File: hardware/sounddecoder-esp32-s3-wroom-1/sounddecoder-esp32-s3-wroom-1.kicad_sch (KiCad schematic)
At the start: 7 parts, among them J1 Input power, U2 IS25WP256D-xM, U3 MAX98357A, U4 DRV8871DDA, U5 LM2594M-5.0, U6 AMS1117-3.3, U7 ESP32-S3-WROOM-1

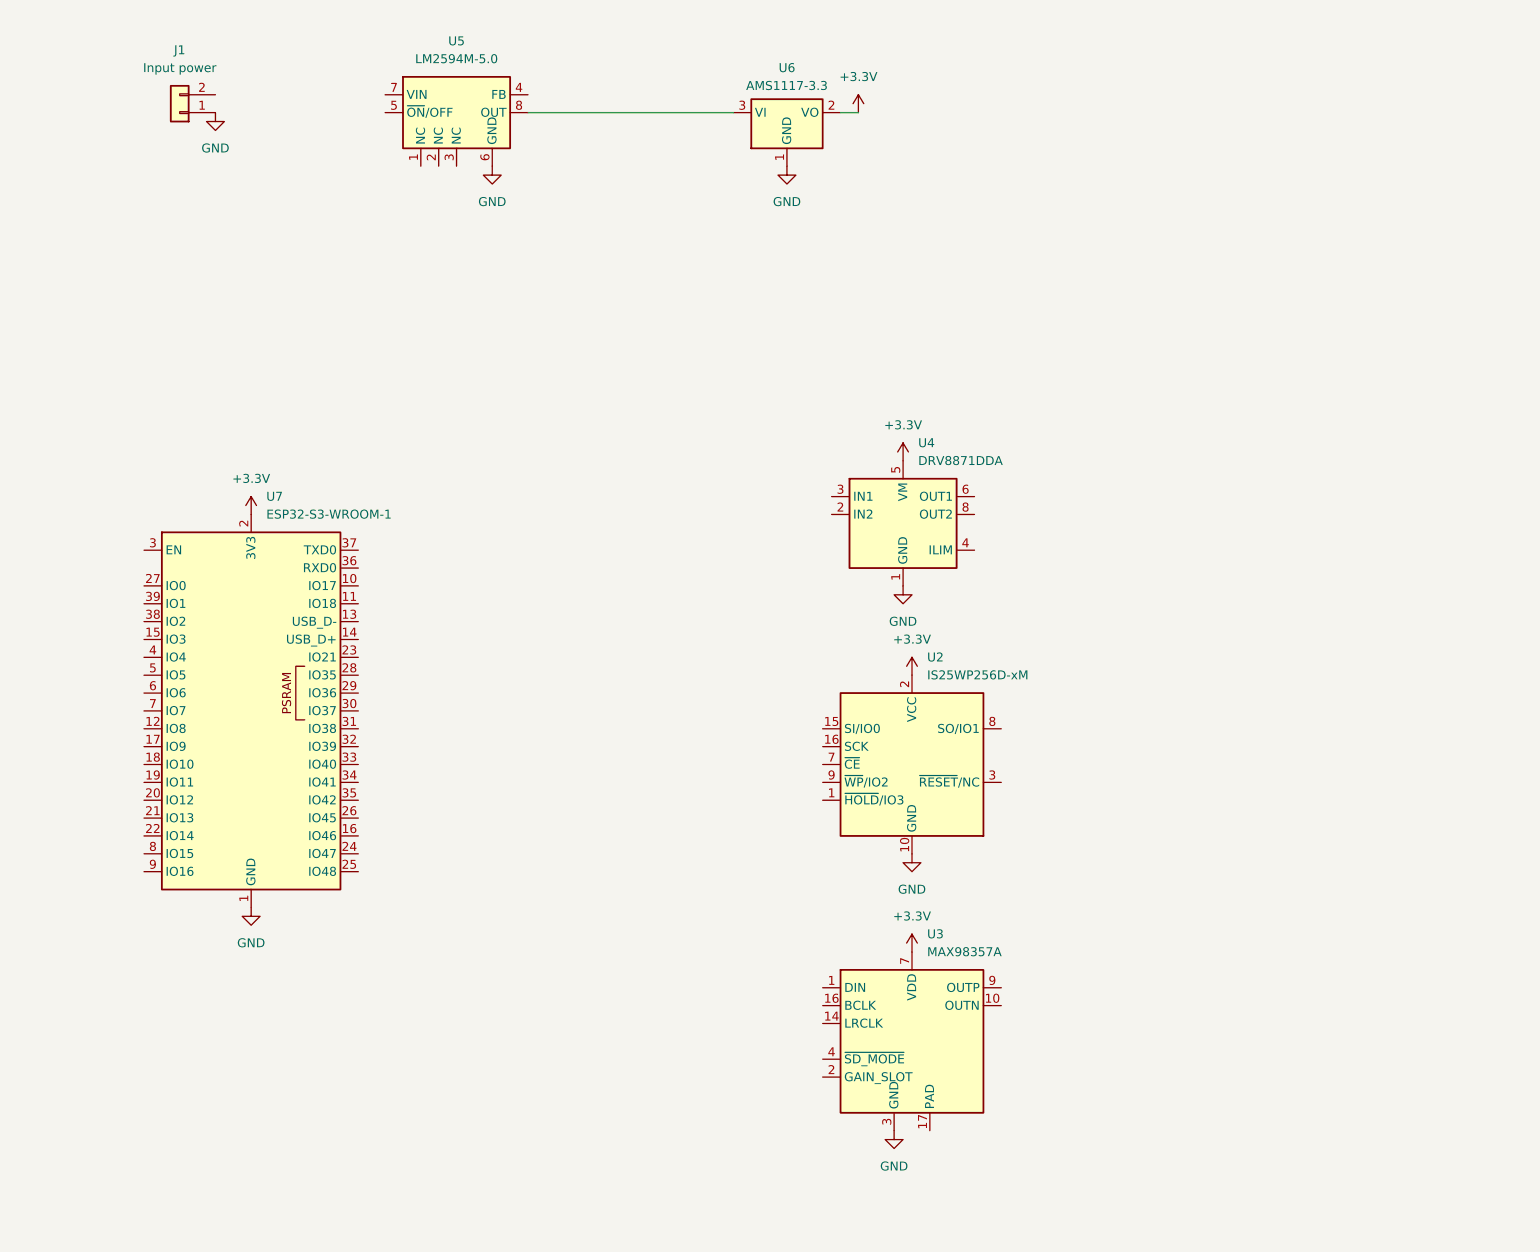
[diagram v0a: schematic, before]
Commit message: Many updates
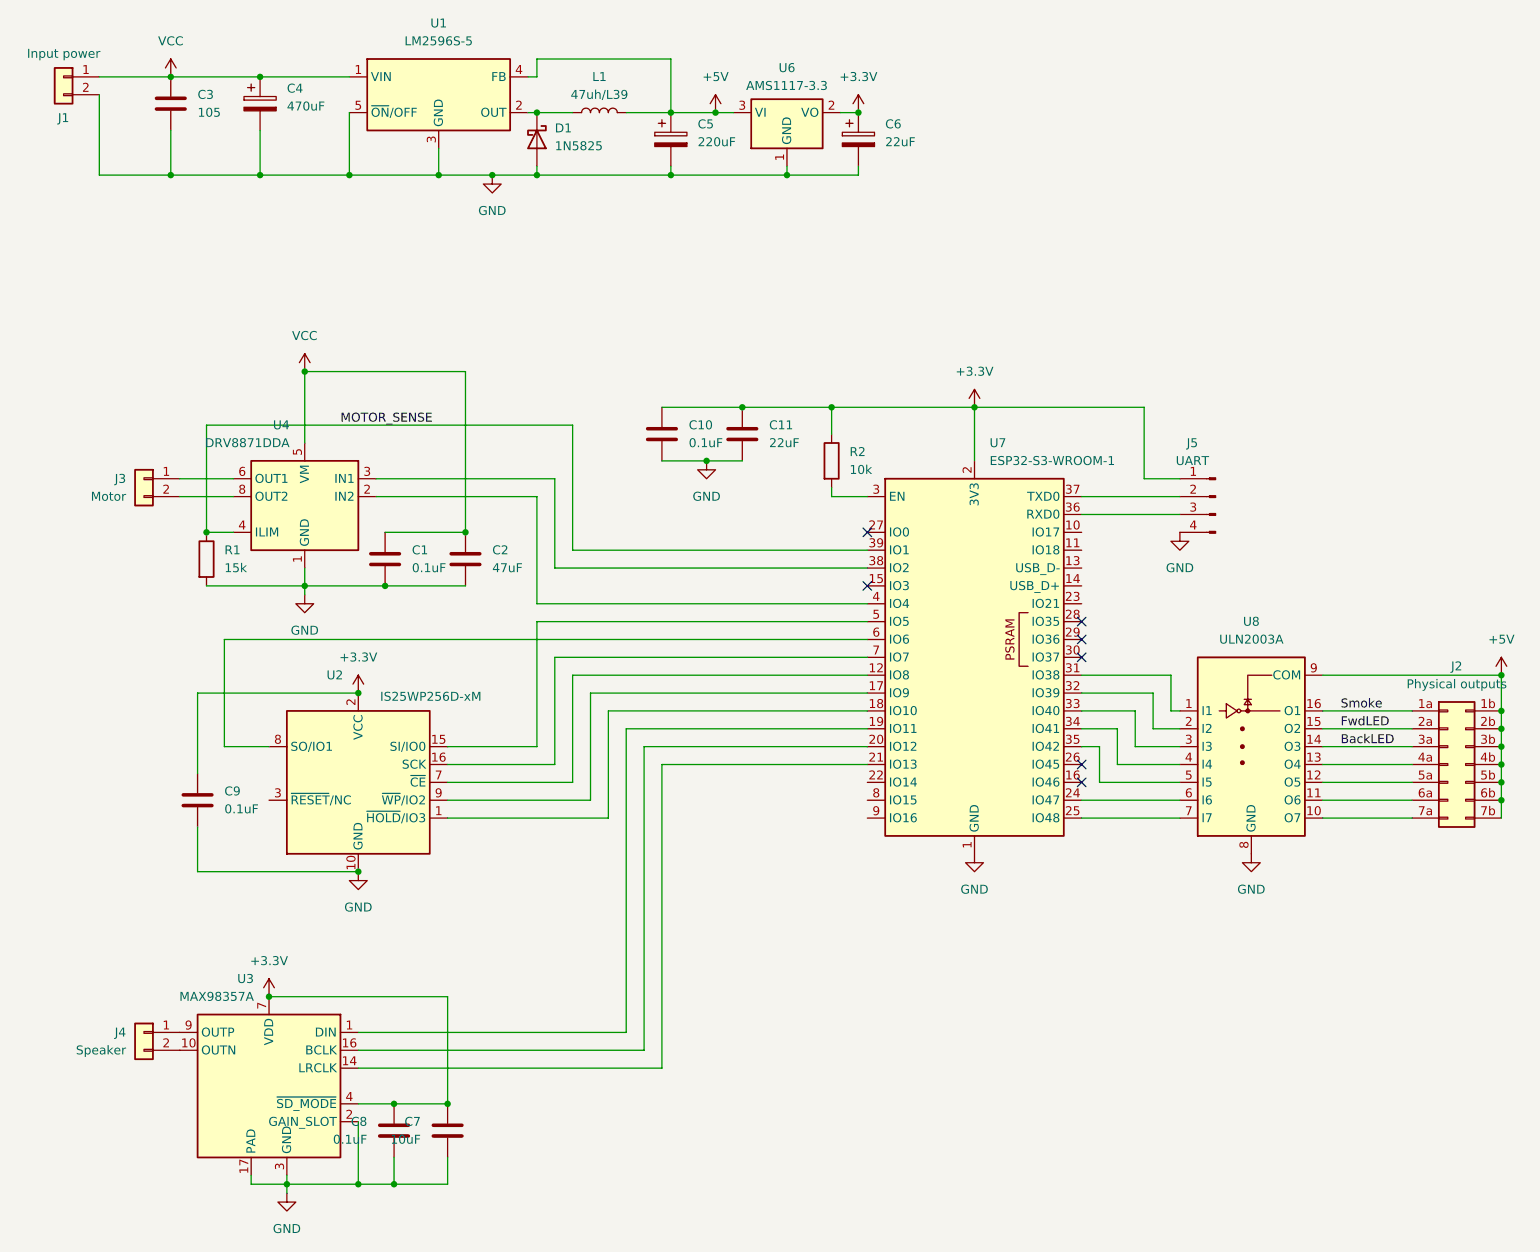
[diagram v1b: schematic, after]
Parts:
- removed U5: LM2594M-5.0, Package_SO:SOIC-8_3.9x4.9mm_P1.27mm, symbol Regulator_Switching:LM2594M-5.0
- added C1, C10, C9: 0.1uF, Capacitor_SMD:C_0805_2012Metric, symbol Device:C
- added C11: 22uF, Capacitor_SMD:C_0805_2012Metric, symbol Device:C
- added C2: 47uF, Capacitor_SMD:C_0805_2012Metric, symbol Device:C
- added C3: 105, symbol Device:C
- added C4: 470uF, symbol Device:C_Polarized
- added C5: 220uF, Capacitor_Tantalum_SMD:CP_EIA-7343-20_Kemet-V_HandSolder, symbol Device:C_Polarized
- added C6: 22uF, Capacitor_Tantalum_SMD:CP_EIA-3216-10_Kemet-I_HandSolder, symbol Device:C_Polarized
- added C7: 10uF, symbol Device:C
- added C8: 0.1uF, symbol Device:C
- added D1: 1N5825, Diode_THT:D_DO-201AD_P15.24mm_Horizontal, symbol Diode:1N5822
- added J2: Physical outputs, symbol Connector_Generic:Conn_02x07_Row_Letter_Last
- added J3: Motor, symbol Connector_Generic:Conn_01x02
- added J4: Speaker, symbol Connector_Generic:Conn_01x02
- added J5: UART, Connector_PinSocket_2.54mm:PinSocket_1x04_P2.54mm_Horizontal, symbol Connector:Conn_01x04_Pin
- added L1: 47uh/L39, Inductor_SMD:L_Bourns_SRP1245A, symbol Device:L
- added R1: 15k, symbol Device:R
- added R2: 10k, symbol Device:R
- added U1: LM2596S-5, Package_TO_SOT_SMD:TO-263-5_TabPin3, symbol Regulator_Switching:LM2596S-5
- added U8: ULN2003A, symbol Transistor_Array:ULN2003A
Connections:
- net +3.3V: now also U3.4 (~{SD_MODE}), C10.1, C11.1, C6.1, C7.1, C8.1, C9.1, J5.1 (Pin_1), R2.1; no longer U4.5 (VM)
- net GND: now also J1.2 (Pin_2), U3.17 (PAD), U3.2 (GAIN_SLOT), C1.2, C10.2, C11.2, C2.2, C3.2, C4.2, C5.2, C6.2, C7.2, C8.2, C9.2, D1.2 (A), J5.4 (Pin_4), R1.2, U1.3 (GND), U1.5 (~{ON}/OFF), U8.8 (GND); no longer J1.1 (Pin_1)
- net at U3.1 (DIN): now also U7.19 (IO11)
- net at U3.10 (OUTN): now also J4.2 (Pin_2)
- net at U3.14 (LRCLK): now also U7.21 (IO13)
- net at U3.16 (BCLK): now also U7.20 (IO12)
- net at U3.9 (OUTP): now also J4.1 (Pin_1)
- net +5V: now reaches U6.3 (VI)
- net +5V: now also C5.1, J2.1b (Pin_1b), J2.2b (Pin_2b), J2.3b (Pin_3b), J2.4b (Pin_4b), J2.5b (Pin_5b), J2.6b (Pin_6b), J2.7b (Pin_7b), L1.2, U1.4 (FB), U8.9 (COM)
- net at U7.12 (IO8): now also U2.7 (~{CE})
- net at U7.17 (IO9): now also U2.9 (~{WP}/IO2)
- net at U7.18 (IO10): now also U2.1 (~{HOLD}/IO3)
- net at U7.24 (IO47): now also U8.6 (I6)
- net at U7.25 (IO48): now also U8.7 (I7)
- net at U7.3 (EN): now also R2.2
- net at U7.31 (IO38): now also U8.1 (I1)
- net at U7.32 (IO39): now also U8.2 (I2)
- net at U7.33 (IO40): now also U8.3 (I3)
- net at U7.34 (IO41): now also U8.4 (I4)
- net at U7.35 (IO42): now also U8.5 (I5)
- net at U7.36 (RXD0): now also J5.3 (Pin_3)
- net at U7.37 (TXD0): now also J5.2 (Pin_2)
- net at U7.38 (IO2): now also U4.3 (IN1)
- net MOTOR_SENSE: now reaches U7.39 (IO1)
- net MOTOR_SENSE: now also U4.4 (ILIM), R1.1
- net at U7.4 (IO4): now also U4.2 (IN2)
- net at U7.5 (IO5): now also U2.15 (SI/IO0)
- net at U7.6 (IO6): now also U2.8 (SO/IO1)
- net at U7.7 (IO7): now also U2.16 (SCK)
- net at U4.6 (OUT1): now also J3.1 (Pin_1)
- net at U4.8 (OUT2): now also J3.2 (Pin_2)
- new net: J2.7a (Pin_7a), U8.10 (O7)
- new net: J2.6a (Pin_6a), U8.11 (O6)
- new net: J2.5a (Pin_5a), U8.12 (O5)
- new net: J2.4a (Pin_4a), U8.13 (O4)
- new net: D1.1 (K), L1.1, U1.2 (OUT)
- new net BackLED: J2.3a (Pin_3a), U8.14 (O3)
- new net FwdLED: J2.2a (Pin_2a), U8.15 (O2)
- new net Smoke: J2.1a (Pin_1a), U8.16 (O1)
- new net VCC: C1.1, C2.1, C3.1, C4.1, J1.1 (Pin_1), U1.1 (VIN), U4.5 (VM)
- no-connect marks 0 -> 7
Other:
- moved on the sheet: J1, U2, U3, U4, U7
